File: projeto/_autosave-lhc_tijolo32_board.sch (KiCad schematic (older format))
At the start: 46 parts, among them J1 USB_A, J2 OLED, J3 JTAG 10pin Connector, J4 CONN_06POLAR, J5 CONN_06POLAR, Q1 MMBT3904, Q2 MMBT3904, SW1 SW_Push, SW2 SW_Push, U1 AP2112K-3.3, U2 CH340G, U3 ESP32-WROOM-32D, U4 AP2112K-3.3, Y1 12MHz 10ppm, Y2 32k 20ppm

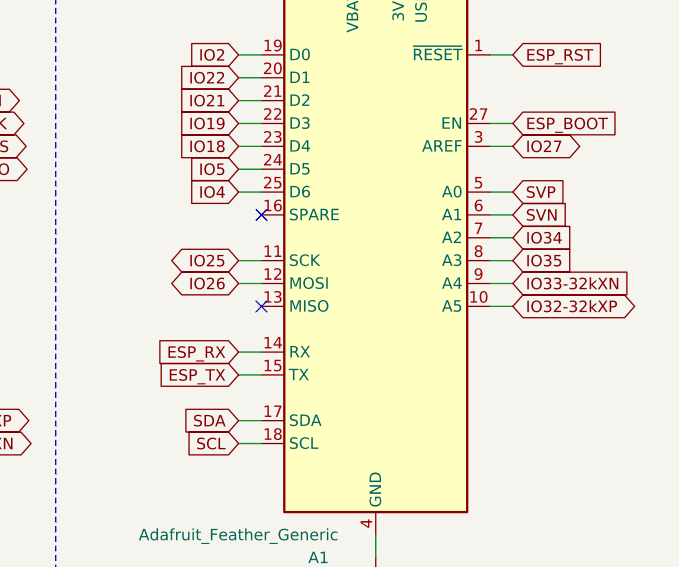
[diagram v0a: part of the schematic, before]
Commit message: Layout improved
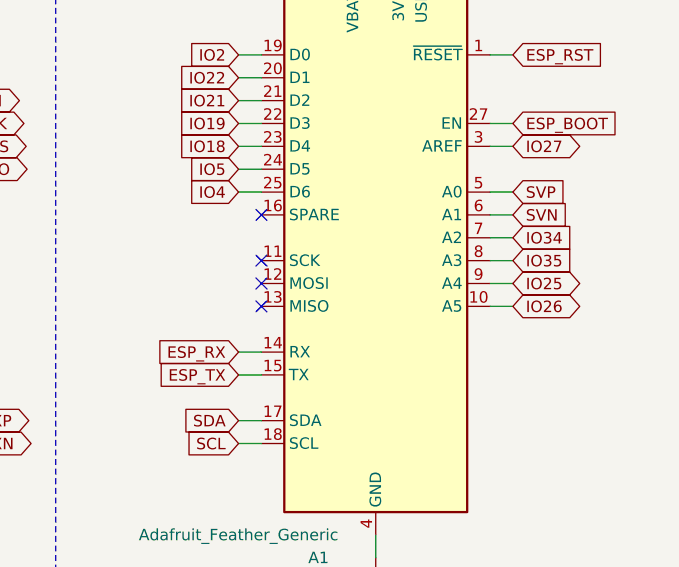
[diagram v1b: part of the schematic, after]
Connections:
- net IO25: now also A1.9 (A4); no longer A1.11 (SCK)
- net IO26: now also A1.10 (A5); no longer A1.12 (MOSI)
- net IO32-32kXP: no longer A1.10 (A5)
- net IO33-32kXN: no longer A1.9 (A4)
- no-connect marks 7 -> 9
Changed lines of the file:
@@
 Wire Notes Line
 	6350 3200 4750 3200
-Text GLabel 10600 2850 2    50   BiDi ~ 0
-IO32-32kXP
-Text GLabel 10600 2750 2    50   Input ~ 0
-IO33-32kXN
 Text GLabel 10600 2550 2    50   Input ~ 0
 IO34
 Text GLabel 10600 2650 2    50   Input ~ 0
 IO35
-Text GLabel 9400 2650 0    50   BiDi ~ 0
+Text GLabel 10600 2750 2    50   BiDi ~ 0
 IO25
-Text GLabel 9400 2750 0    50   BiDi ~ 0
+Text GLabel 10600 2850 2    50   BiDi ~ 0
 IO26
 Text GLabel 10600 2150 2    50   BiDi ~ 0
@@
 	10500 2650 10600 2650
 Wire Wire Line
-	10500 2750 10600 2750
-Wire Wire Line
-	10500 2850 10600 2850
-Wire Wire Line
-	9400 2650 9500 2650
-Wire Wire Line
-	9400 2750 9500 2750
-Wire Wire Line
 	10000 3950 10000 3850
 $Comp
@@
 NoConn ~ 9500 2450
 NoConn ~ 9500 2850
+Wire Wire Line
+	10500 2750 10600 2750
+Wire Wire Line
+	10500 2850 10600 2850
+NoConn ~ 9500 2750
+NoConn ~ 9500 2650
 $EndSCHEMATC
